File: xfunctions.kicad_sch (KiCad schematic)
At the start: 34 parts, among them SW0 SW_Push, SW1 SW_Push, SW10 SW_Push, SW11 SW_Push, SW12 SW_Push, SW13 SW_Push, SW14 SW_Push, SW15 SW_Push, SW2 SW_Push, SW3 SW_Push, SW4 SW_Push, SW5 SW_Push, SW6 SW_Push, SW7 SW_Push, SW8 SW_Push, SW9 SW_Push, U1 ProMicro, U2 74HC4051

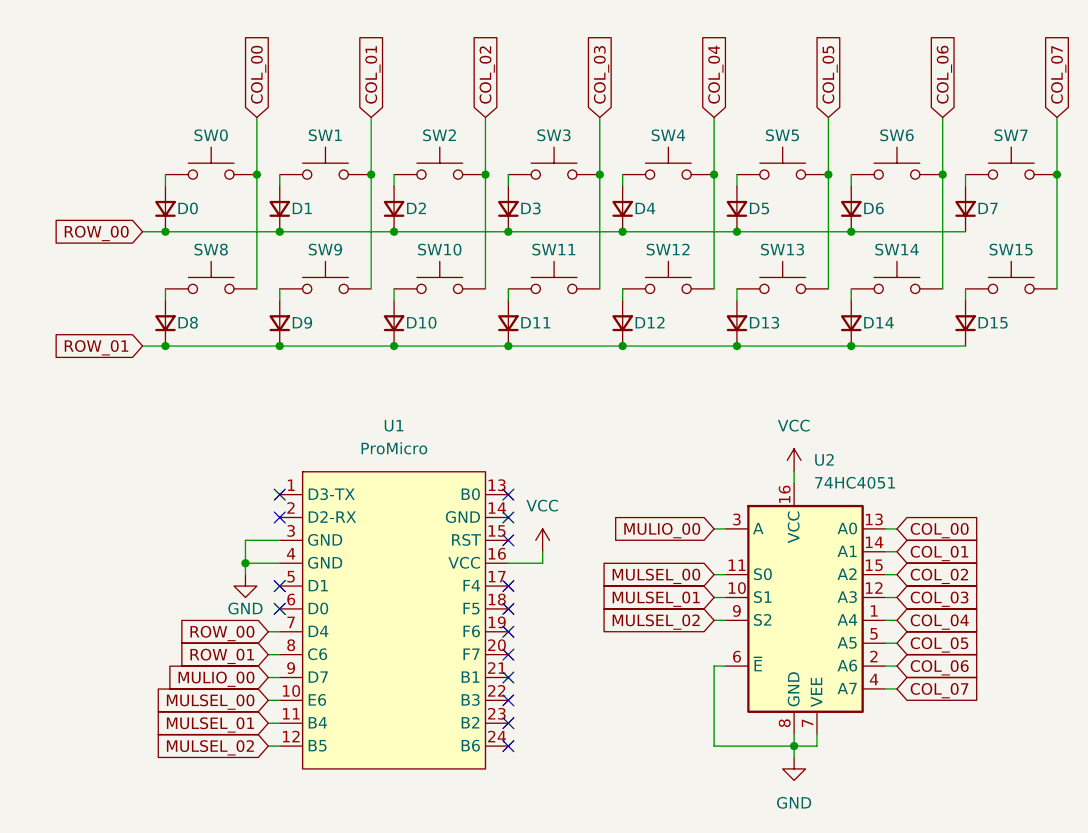
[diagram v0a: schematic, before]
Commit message: PCB 작성 완료
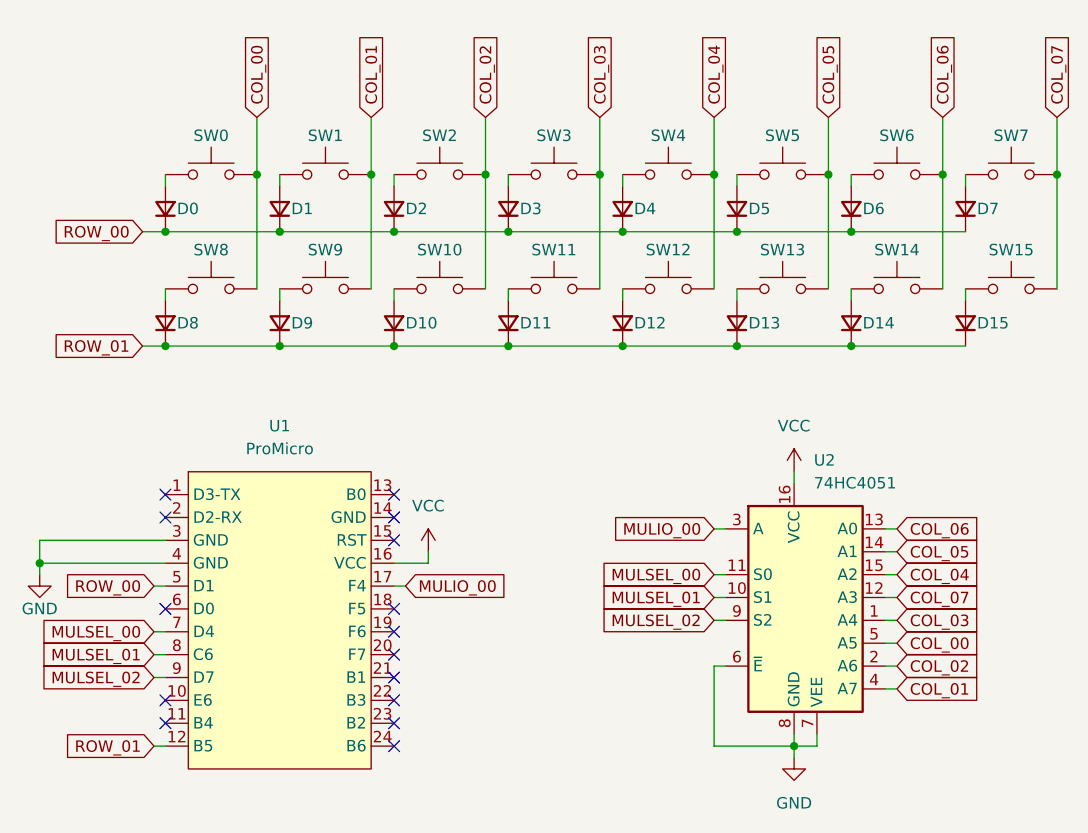
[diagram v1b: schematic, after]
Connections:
- net COL_00: now also U2.5 (A5); no longer U2.13 (A0)
- net COL_01: now also U2.4 (A7); no longer U2.14 (A1)
- net COL_02: now also U2.2 (A6); no longer U2.15 (A2)
- net COL_03: now also U2.1 (A4); no longer U2.12 (A3)
- net COL_04: now also U2.15 (A2); no longer U2.1 (A4)
- net COL_05: now also U2.14 (A1); no longer U2.5 (A5)
- net COL_06: now also U2.13 (A0); no longer U2.2 (A6)
- net COL_07: now also U2.12 (A3); no longer U2.4 (A7)
- net MULIO_00: now also U1.17 (F4); no longer U1.9 (D7)
- net MULSEL_00: now also U1.7 (D4); no longer U1.10 (E6)
- net MULSEL_01: now also U1.8 (C6); no longer U1.11 (B4)
- net MULSEL_02: now also U1.9 (D7); no longer U1.12 (B5)
- net ROW_00: now also U1.5 (D1); no longer U1.7 (D4)
- net ROW_01: now also U1.12 (B5); no longer U1.8 (C6)
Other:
- moved on the sheet: U1
